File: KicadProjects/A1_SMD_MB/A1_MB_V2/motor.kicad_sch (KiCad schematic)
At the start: 18 parts, among them U3 TMC2209-LA

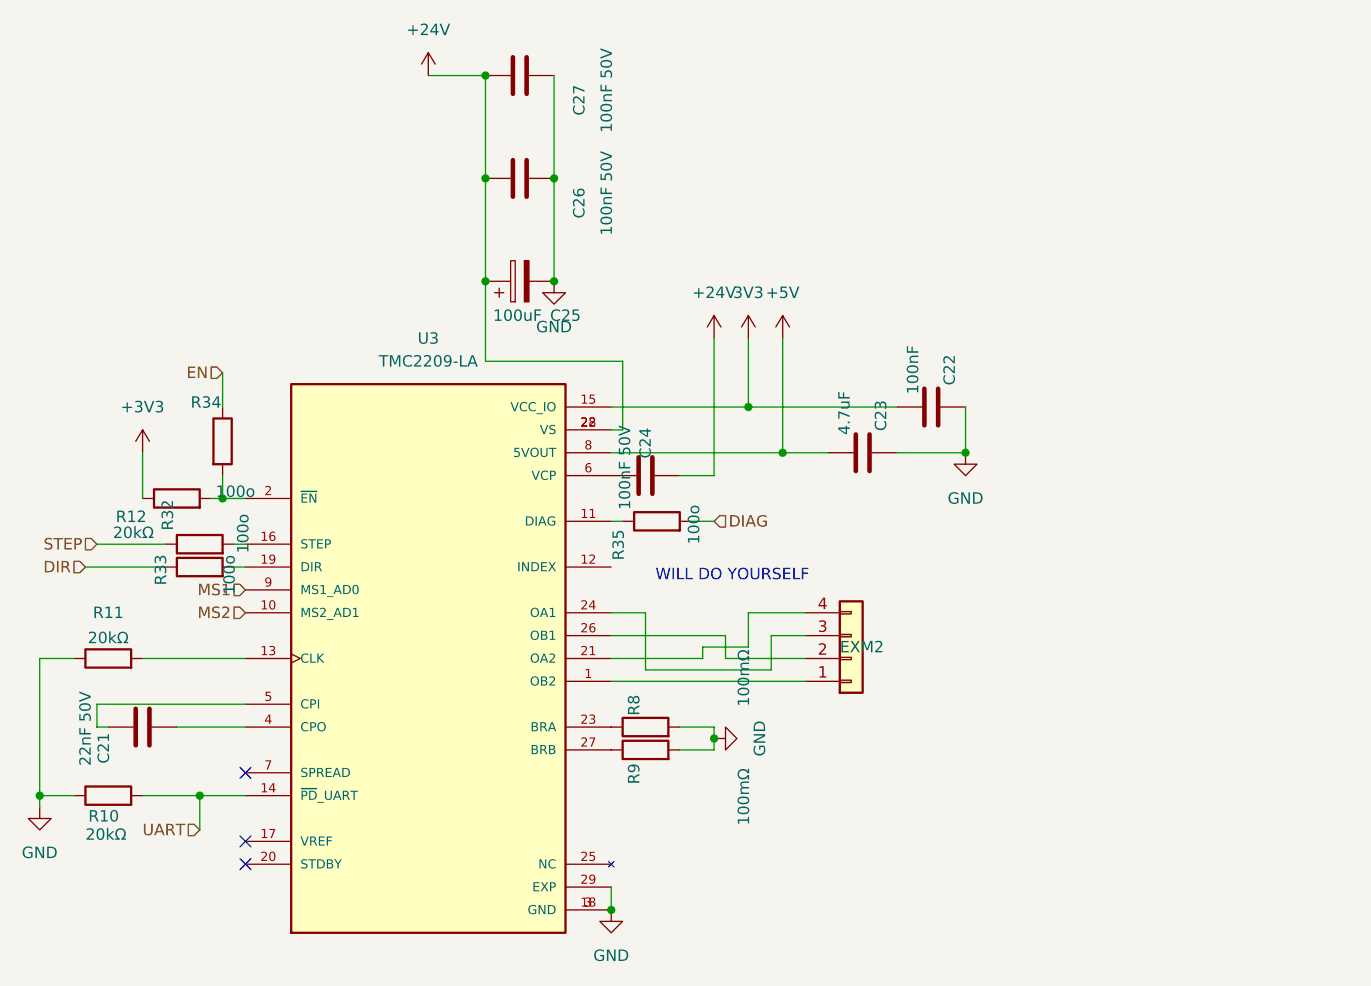
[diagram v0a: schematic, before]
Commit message: e
e
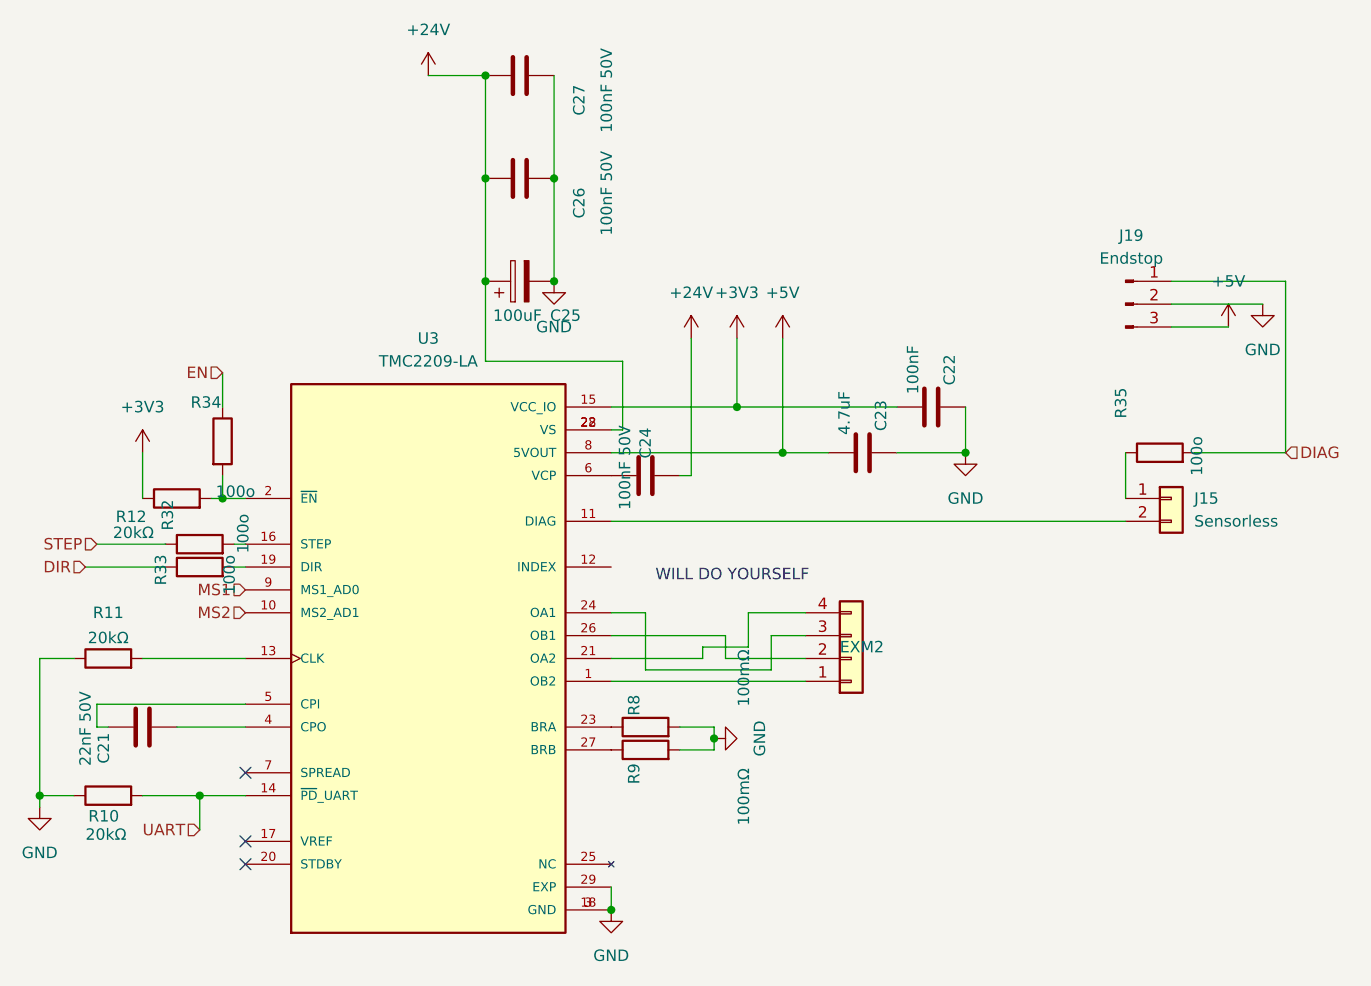
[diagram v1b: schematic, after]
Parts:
- added J15: Sensorless, Connector_PinHeader_2.54mm:PinHeader_1x02_P2.54mm_Vertical, symbol Connector_Generic:Conn_01x02
- added J19: Endstop, Connector_JST:JST_XH_B3B-XH-A_1x03_P2.50mm_Vertical, symbol Connector:Conn_01x03_Pin
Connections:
- net 3V3 is gone; now on net +3V3: C22.2, U3.15 (VCC_IO)
- net +5V: now also J19.3 (Pin_3)
- net DIAG: now also J19.1 (Pin_1)
- net GND: now also J19.2 (Pin_2)
- net at R35.1: now also J15.1 (Pin_1); no longer U3.11 (DIAG)
- new net: J15.2 (Pin_2), U3.11 (DIAG)
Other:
- moved on the sheet: R35
